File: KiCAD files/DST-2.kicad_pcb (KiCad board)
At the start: 2 copper layers, 50 x 50 mm, 53 parts, among them J1 FTSW, J4 Pot_Dis, J5 Pot_Tone, J6 Pot_Vol, Q1 2N3904, Q2 2N3904, Q3 2N3904, U1 TL072

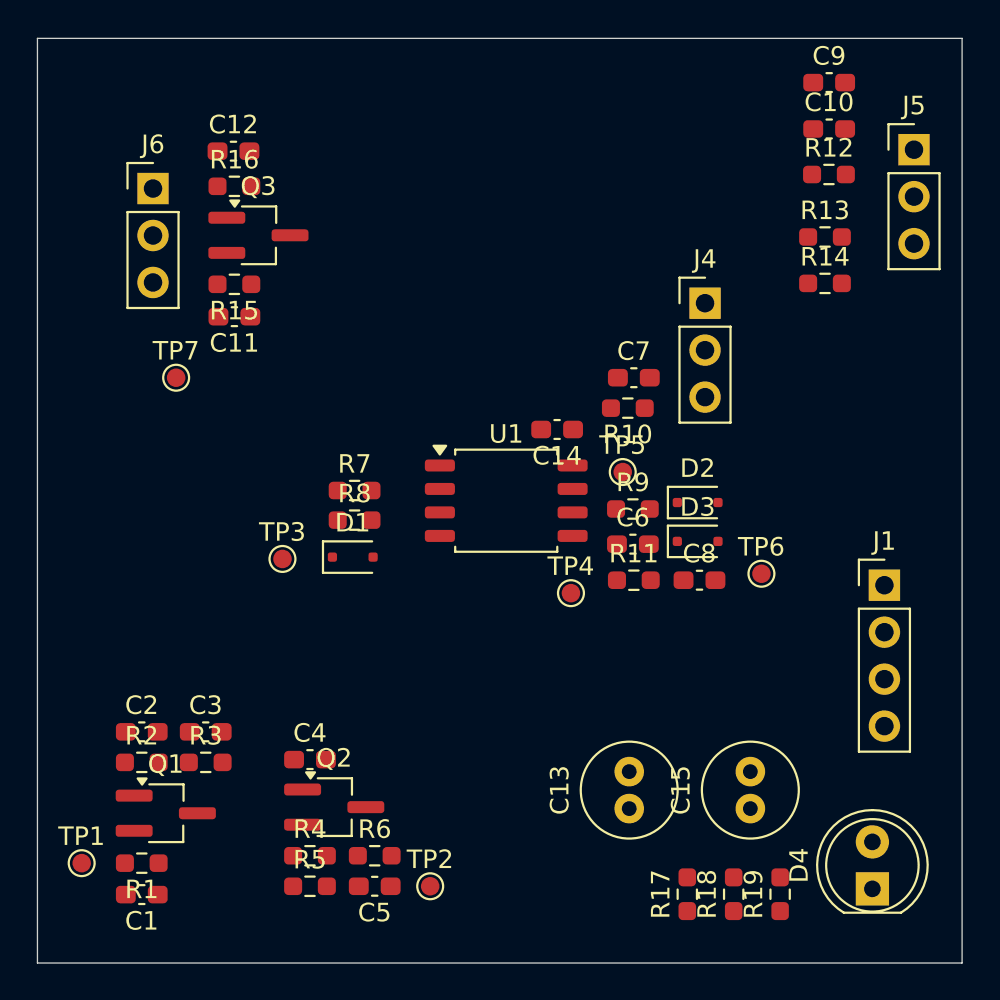
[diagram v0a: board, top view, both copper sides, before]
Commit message: Finished PCB design
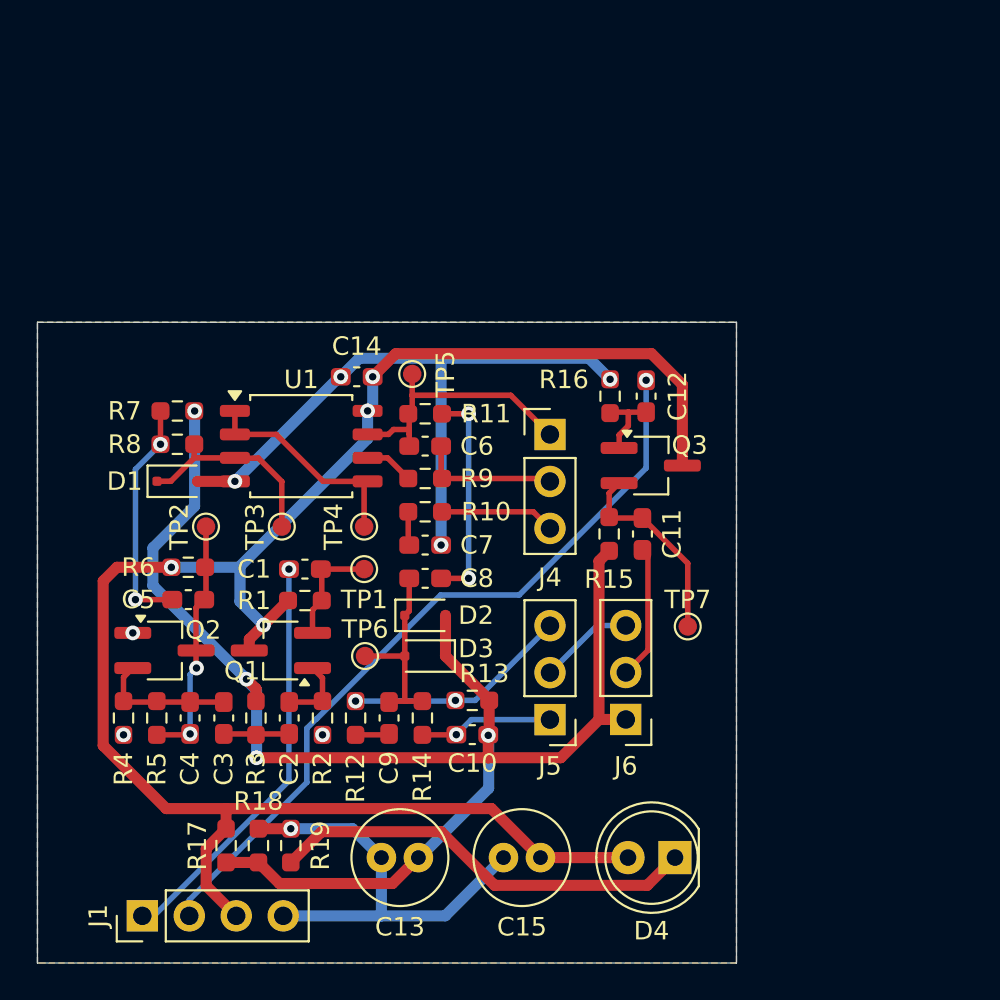
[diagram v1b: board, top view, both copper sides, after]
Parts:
- moved J1 43.9 mm to (130.7, 122.5), turned to 90 degrees
- moved C9 41.8 mm to (144.0, 111.8), turned to -90 degrees
- moved R12 39.0 mm to (142.2, 111.8), turned to 90 degrees
- moved J6 38.4 mm to (156.8, 111.8), turned to 180 degrees
- moved C10 38.0 mm to (148.5, 112.7), turned to 180 degrees
- moved J5 36.6 mm to (152.7, 111.8), turned to 180 degrees
- moved R14 32.0 mm to (145.8, 111.8), turned to -90 degrees
- moved R13 31.5 mm to (148.5, 110.8)
- moved TP7 30.8 mm to (160.2, 106.8)
- moved R19 26.6 mm to (138.7, 118.7)
- moved C12 26.0 mm to (157.9, 94.3), turned to 90 degrees
- moved R18 25.8 mm to (136.9, 118.7)
- moved R17 25.1 mm to (135.2, 118.7), turned to -90 degrees
- moved C11 25.0 mm to (157.7, 101.8), turned to 90 degrees
- moved Q3 24.6 mm to (158.2, 98.1)
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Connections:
- C1 pad 1: in_p -> IN_P
- C12 pad 2: out_p -> OUT_P
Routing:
- net +9V: track 0.00 -> 97.2 mm, vias 0 -> 4
- net +4,5v: track 0.00 -> 82.0 mm, vias 0 -> 4
- net GND: track 0.00 -> 59.3 mm, vias 0 -> 8
- net OUT_P: track 0.00 -> 41.7 mm, vias 0 -> 1
- net Net-(D4-K): track 0.00 -> 23.3 mm
- net IN_P: track 0.00 -> 22.4 mm, vias 0 -> 1
- net Net-(J4-Pin_1): track 0.00 -> 14.7 mm
- net Net-(Q2-C): track 0.00 -> 13.4 mm, vias 0 -> 2
- net Net-(C5-Pad2): track 0.00 -> 12.8 mm, vias 0 -> 2
- net Net-(J5-Pin_3): track 0.00 -> 12.2 mm, vias 0 -> 2
- net Net-(U1A--): track 0.00 -> 12.0 mm
- net Net-(C8-Pad1): track 0.00 -> 11.8 mm, vias 0 -> 2
- net Net-(D1-K): track 0.00 -> 11.0 mm
- net Net-(Q3-B): track 0.00 -> 10.8 mm
- net Net-(D2-K): track 0.00 -> 10.7 mm
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- added copper zone on B.Cu, net GND
- added copper zone on F.Cu, net GND
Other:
- board size 50 x 50 mm -> 37.8 x 34.7 mm
